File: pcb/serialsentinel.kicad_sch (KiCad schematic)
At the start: 39 parts, among them J2 Bus_PCI_Express_x1, J3 REL1, J4 REL1, J5 REL2, J6 REL2, K2 G6K-2F-Y DC3, K3 G6K-2F-Y DC3, Q2 MMBT3904, Q3 MMBT3904, Q4 MMBT3904, Q5 MMBT3904, SW1 RESET, U1 CH382L, U2 XC6206P182MR, U3 ESP32-C3-WROOM-02U

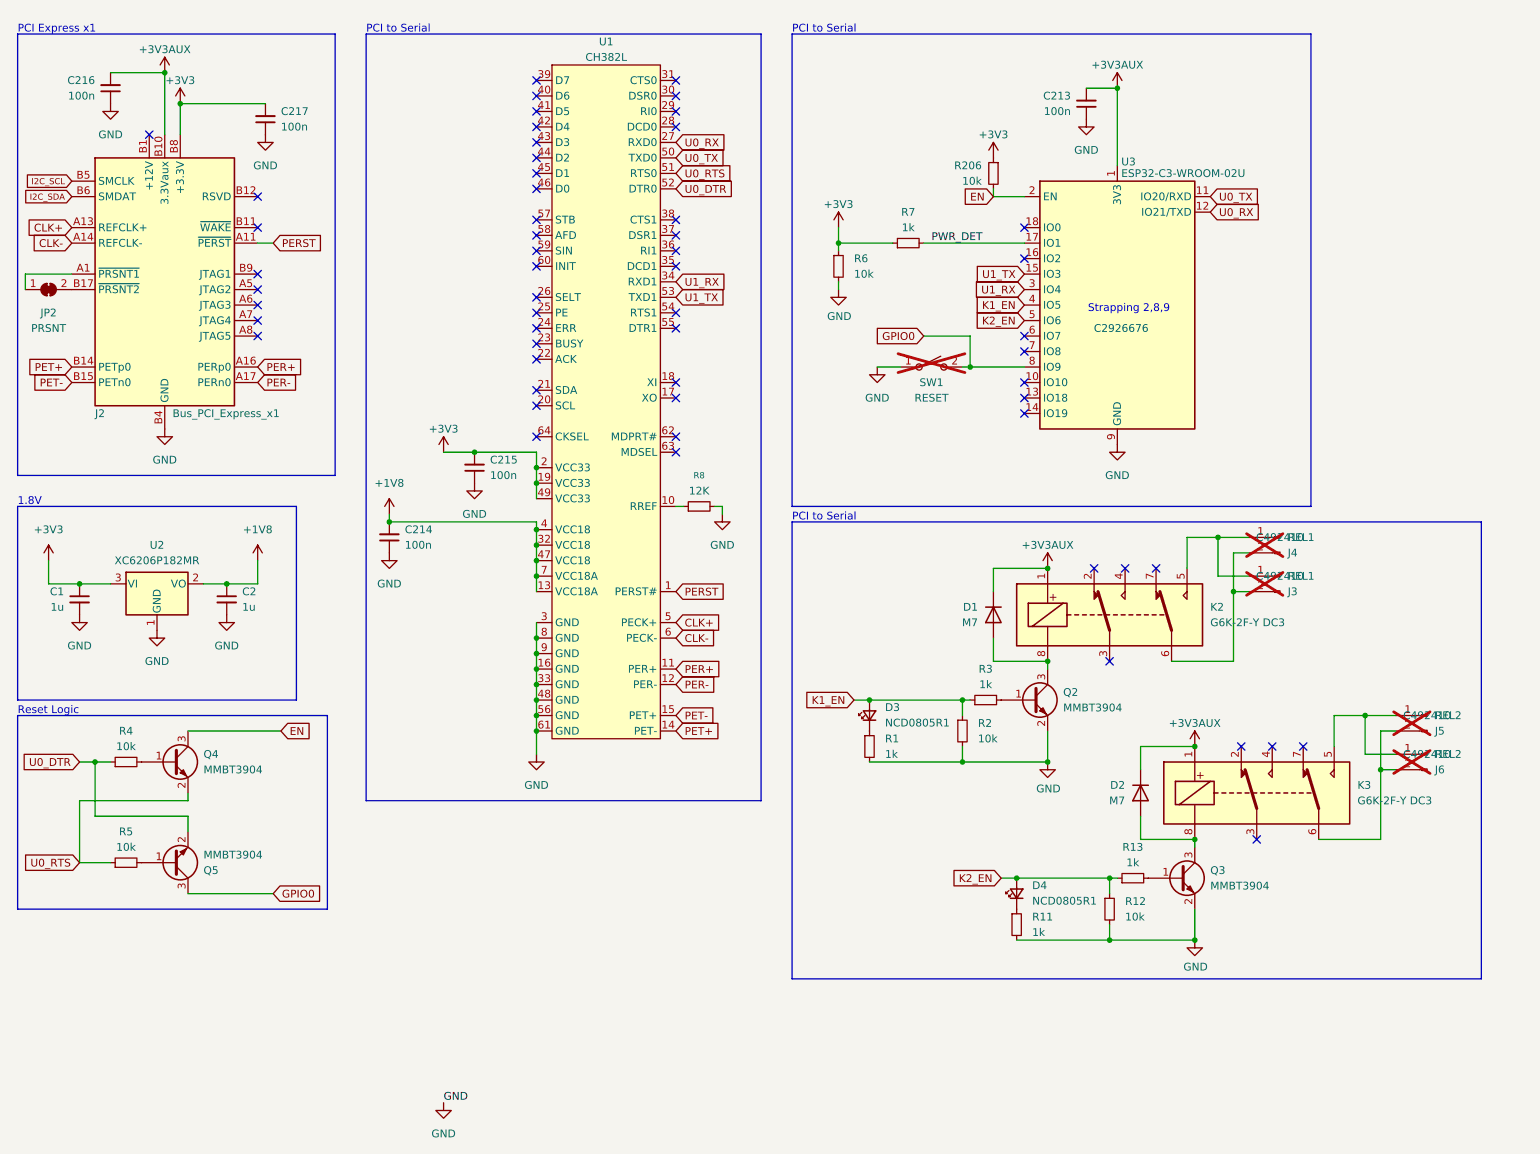
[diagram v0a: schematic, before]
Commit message: tweaks
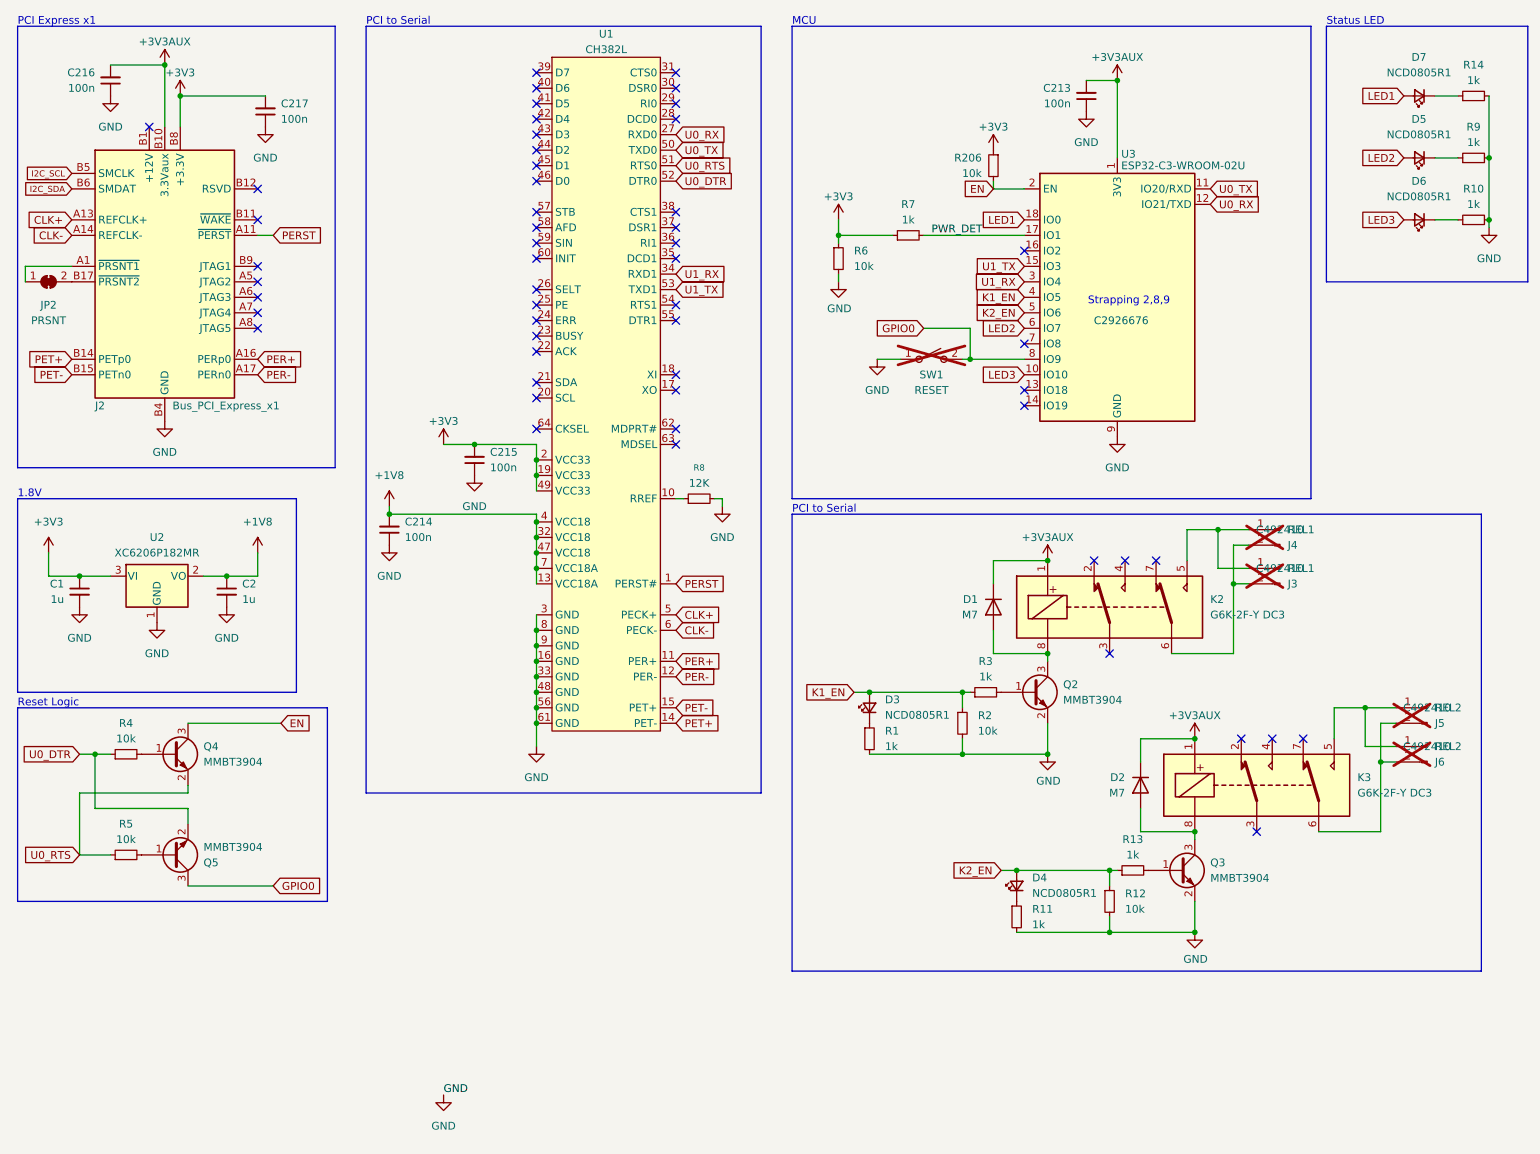
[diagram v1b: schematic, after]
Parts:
- added D5, D6, D7: NCD0805R1, LED_SMD:LED_0805_2012Metric, symbol Device:LED_Small
- added R10, R14, R9: 1k, Resistor_SMD:R_0402_1005Metric, symbol Device:R_Small
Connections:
- net GND: now also R10.2, R14.2, R9.2
- net LED3: now reaches U3.10 (IO10)
- net LED3: now also D6.2 (A)
- net LED1: now reaches U3.18 (IO0)
- net LED1: now also D7.2 (A)
- net LED2: now reaches U3.6 (IO7)
- net LED2: now also D5.2 (A)
- new net: D6.1 (K), R10.1
- new net: D5.1 (K), R9.1
- new net: D7.1 (K), R14.1
- no-connect marks 57 -> 54
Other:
- note added: "MCU"
- note added: "Status LED"
- moved on the sheet: C1, C2, C213, C214, C215, C216, C217, D1, D2, D3, D4, J2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

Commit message: final tweaks
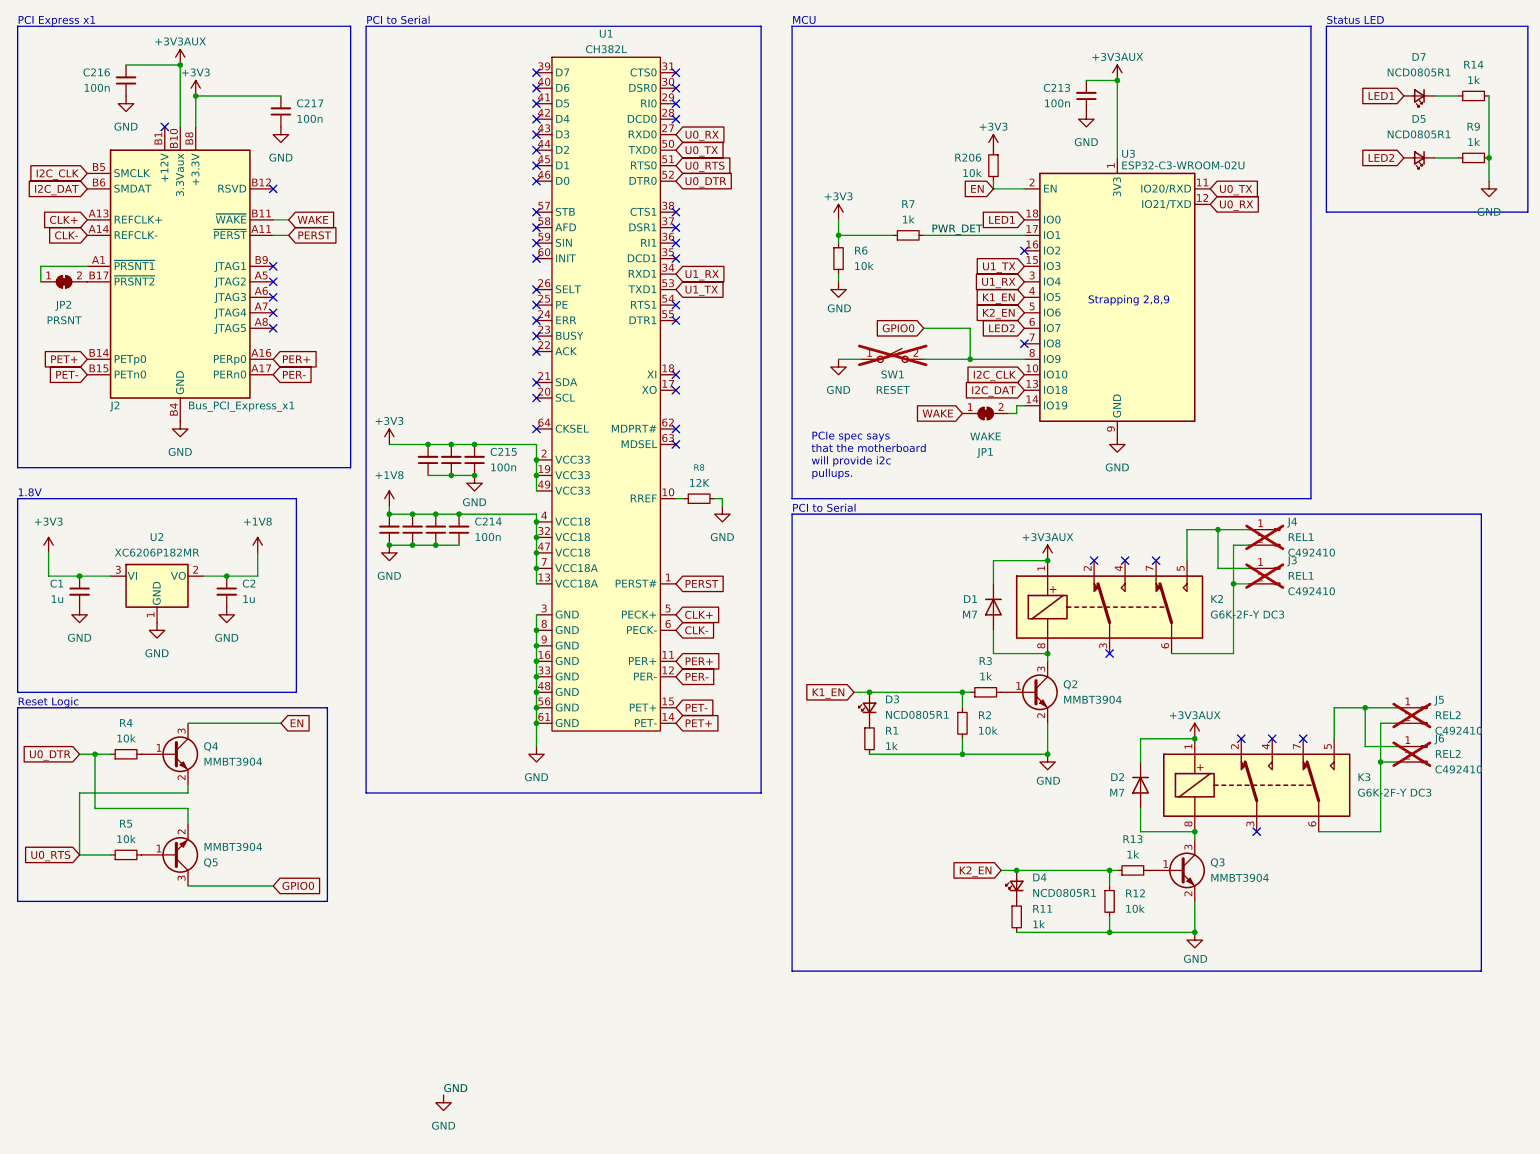
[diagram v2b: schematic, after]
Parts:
- removed D6: NCD0805R1, LED_SMD:LED_0805_2012Metric, symbol Device:LED_Small
- removed R10: 1k, Resistor_SMD:R_0402_1005Metric, symbol Device:R_Small
- added C4, C5, C6, C7, C8: 100n, Capacitor_SMD:C_0402_1005Metric, symbol Device:C_Small
- added JP1: WAKE, Jumper:SolderJumper-2_P1.3mm_Bridged_RoundedPad1.0x1.5mm, symbol Jumper:SolderJumper_2_Bridged
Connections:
- net I2C_SDA is gone; now on net I2C_DAT: J2.B6 (SMDAT)
- net LED3 is gone; now on net I2C_CLK: U3.10 (IO10)
- net +1V8: now also C4.2, C6.2, C8.2
- net +3V3: now also C5.2, C7.2
- net GND: now also C4.1, C5.1, C6.1, C7.1, C8.1
- net I2C_DAT: now reaches U3.13 (IO18)
- net at U3.14 (IO19): now also JP1.2 (B)
- net WAKE: now reaches J2.B11 (~{WAKE})
- net WAKE: now also JP1.1 (A)
- net I2C_SCL renamed I2C_CLK
- no-connect marks 54 -> 51
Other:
- note added: "PCIe spec says that the motherboard will provide i2c pullups."
- moved on the sheet: C214, C216, C217, J2, JP2, SW1
